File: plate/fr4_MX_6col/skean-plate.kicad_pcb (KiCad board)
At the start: 2 copper layers, 134.2 x 95.3 mm, 30 parts, among them K1 KEYSW, K11 KEYSW, K12 KEYSW, K13 KEYSW, K14 KEYSW, K15 KEYSW, K16 KEYSW, K17 KEYSW, K18 KEYSW, K19 KEYSW, K2 KEYSW, K20 KEYSW, K21 KEYSW, K22 KEYSW, K3 KEYSW, K4 KEYSW, K5 KEYSW, K6 KEYSW, K7 KEYSW, K8 KEYSW, K9 KEYSW

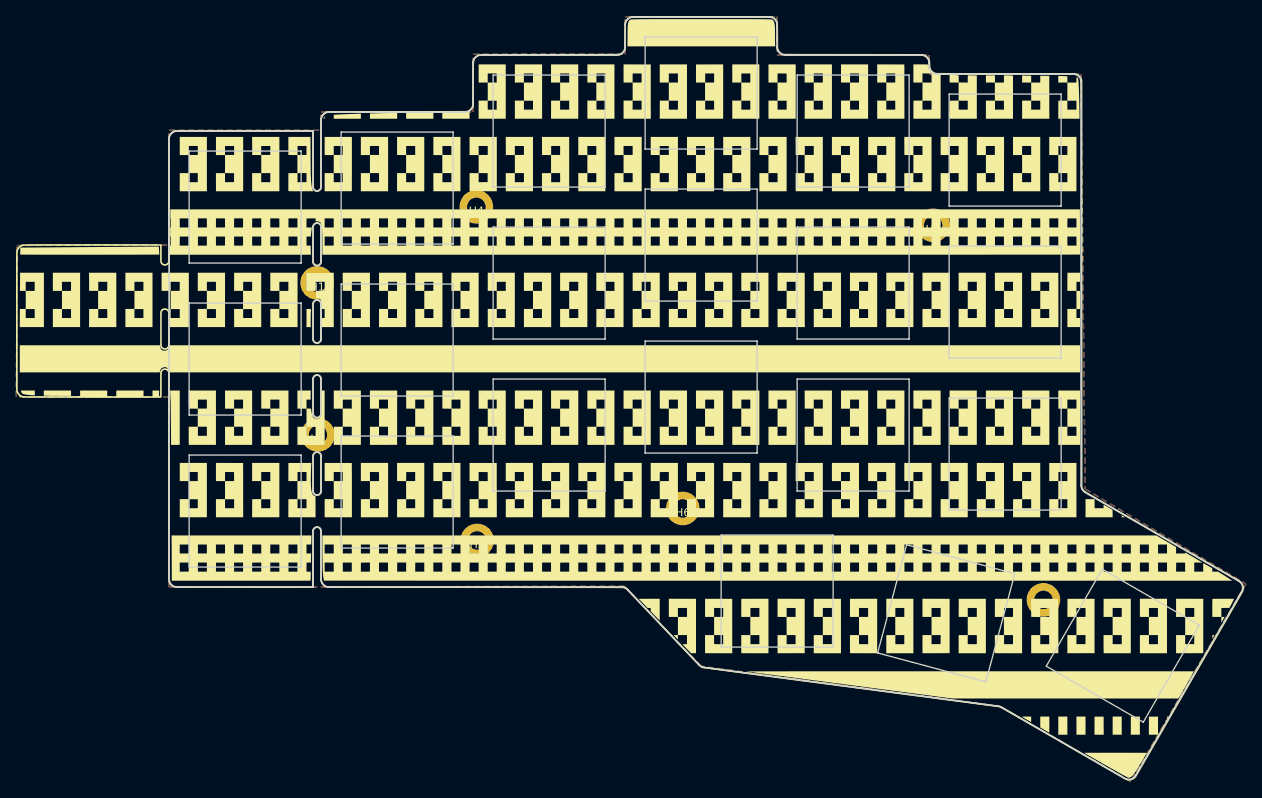
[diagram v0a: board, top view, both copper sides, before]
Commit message: V0.3 case files
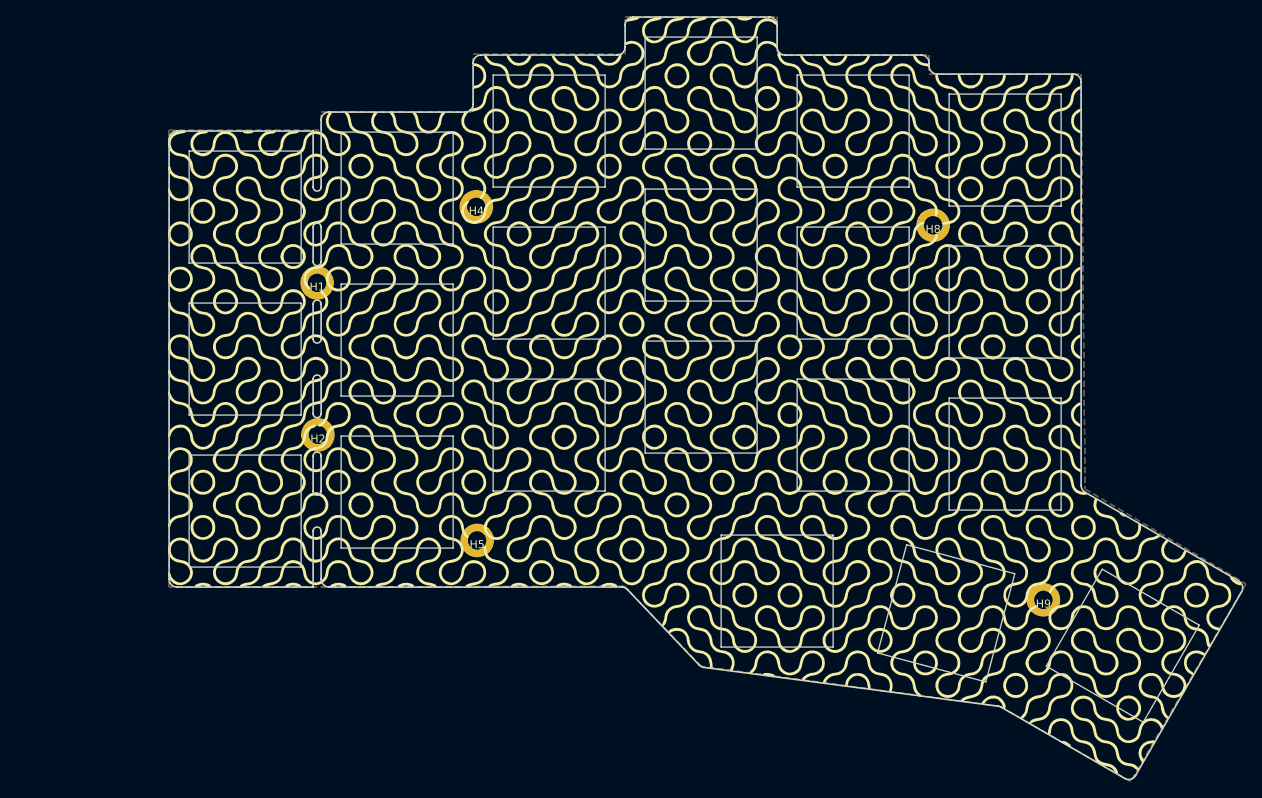
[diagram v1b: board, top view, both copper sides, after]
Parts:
- removed the G*** at (90.8, 62.0) (x2)
- removed H6: MountingHole, kbd:M2_Hole_TH
- added G***: LOGO, Silks:skean_truchet_6col, F.Cu at (100.1, 61.6)
- added G***: LOGO, Silks:skean_truchet_6col_back, F.Cu at (100.1, 61.6)
